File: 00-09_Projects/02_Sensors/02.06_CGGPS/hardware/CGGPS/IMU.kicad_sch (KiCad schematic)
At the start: 12 parts, among them U3 BNO086, Y1 Crystal_GND24

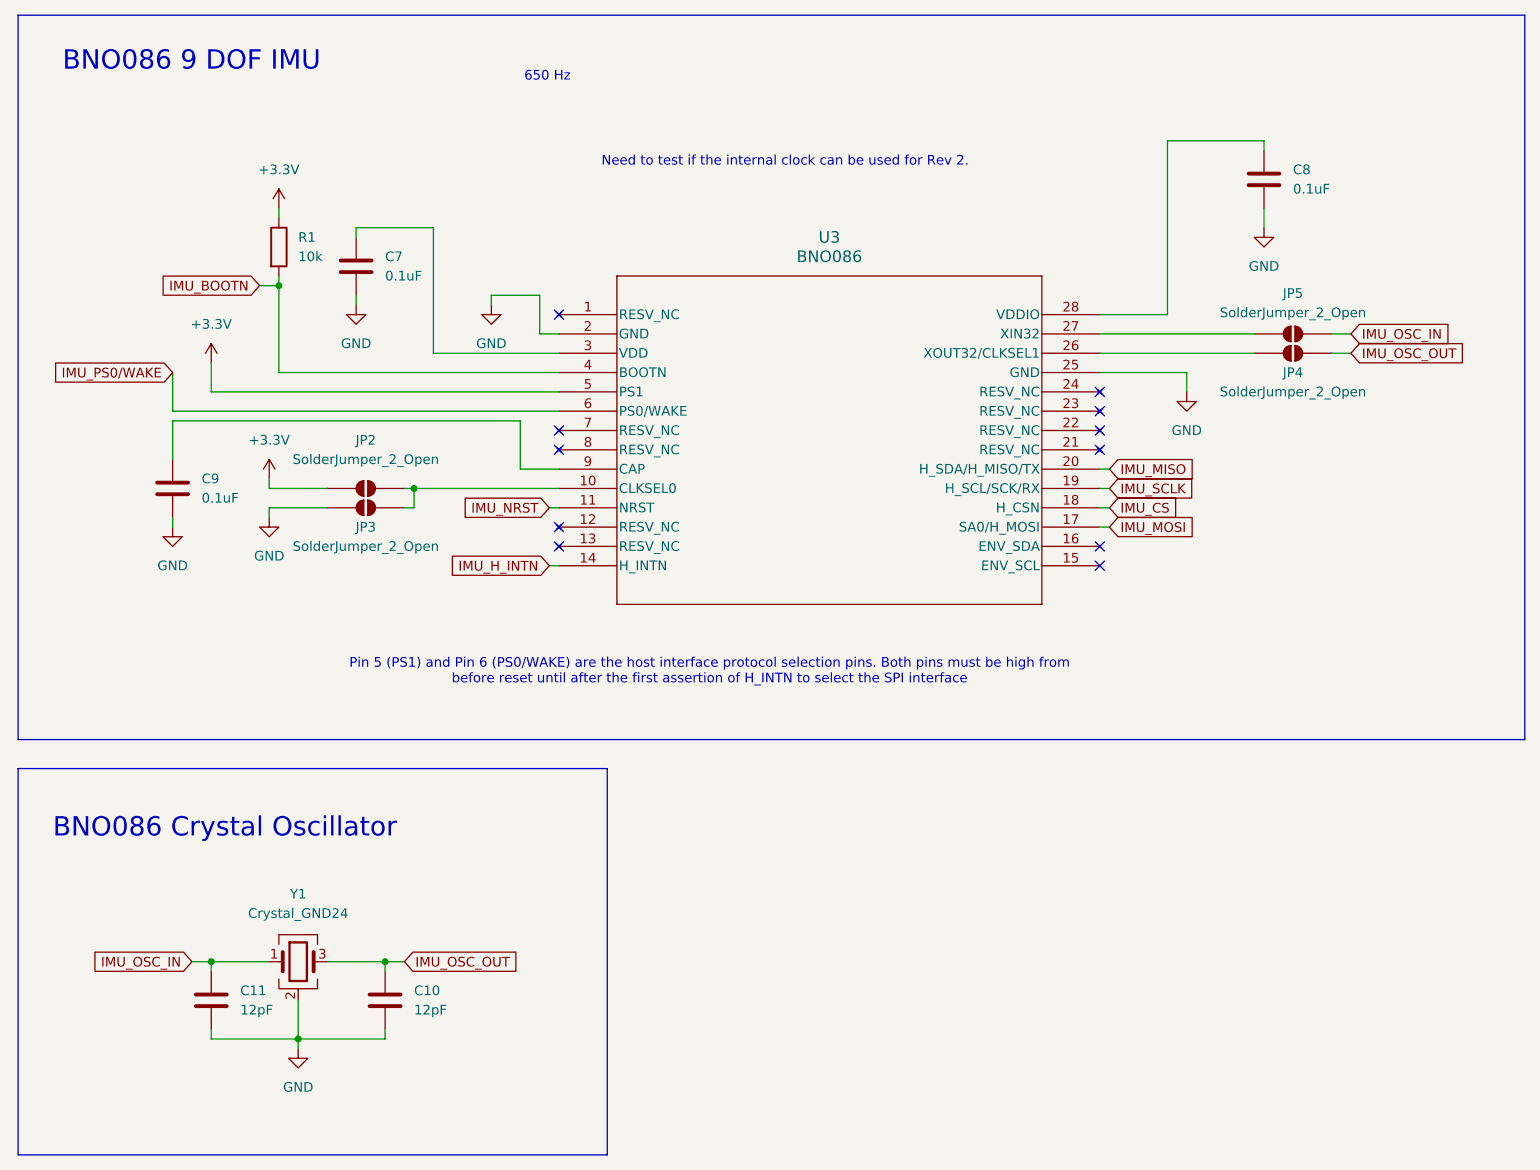
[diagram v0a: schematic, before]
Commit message: wip
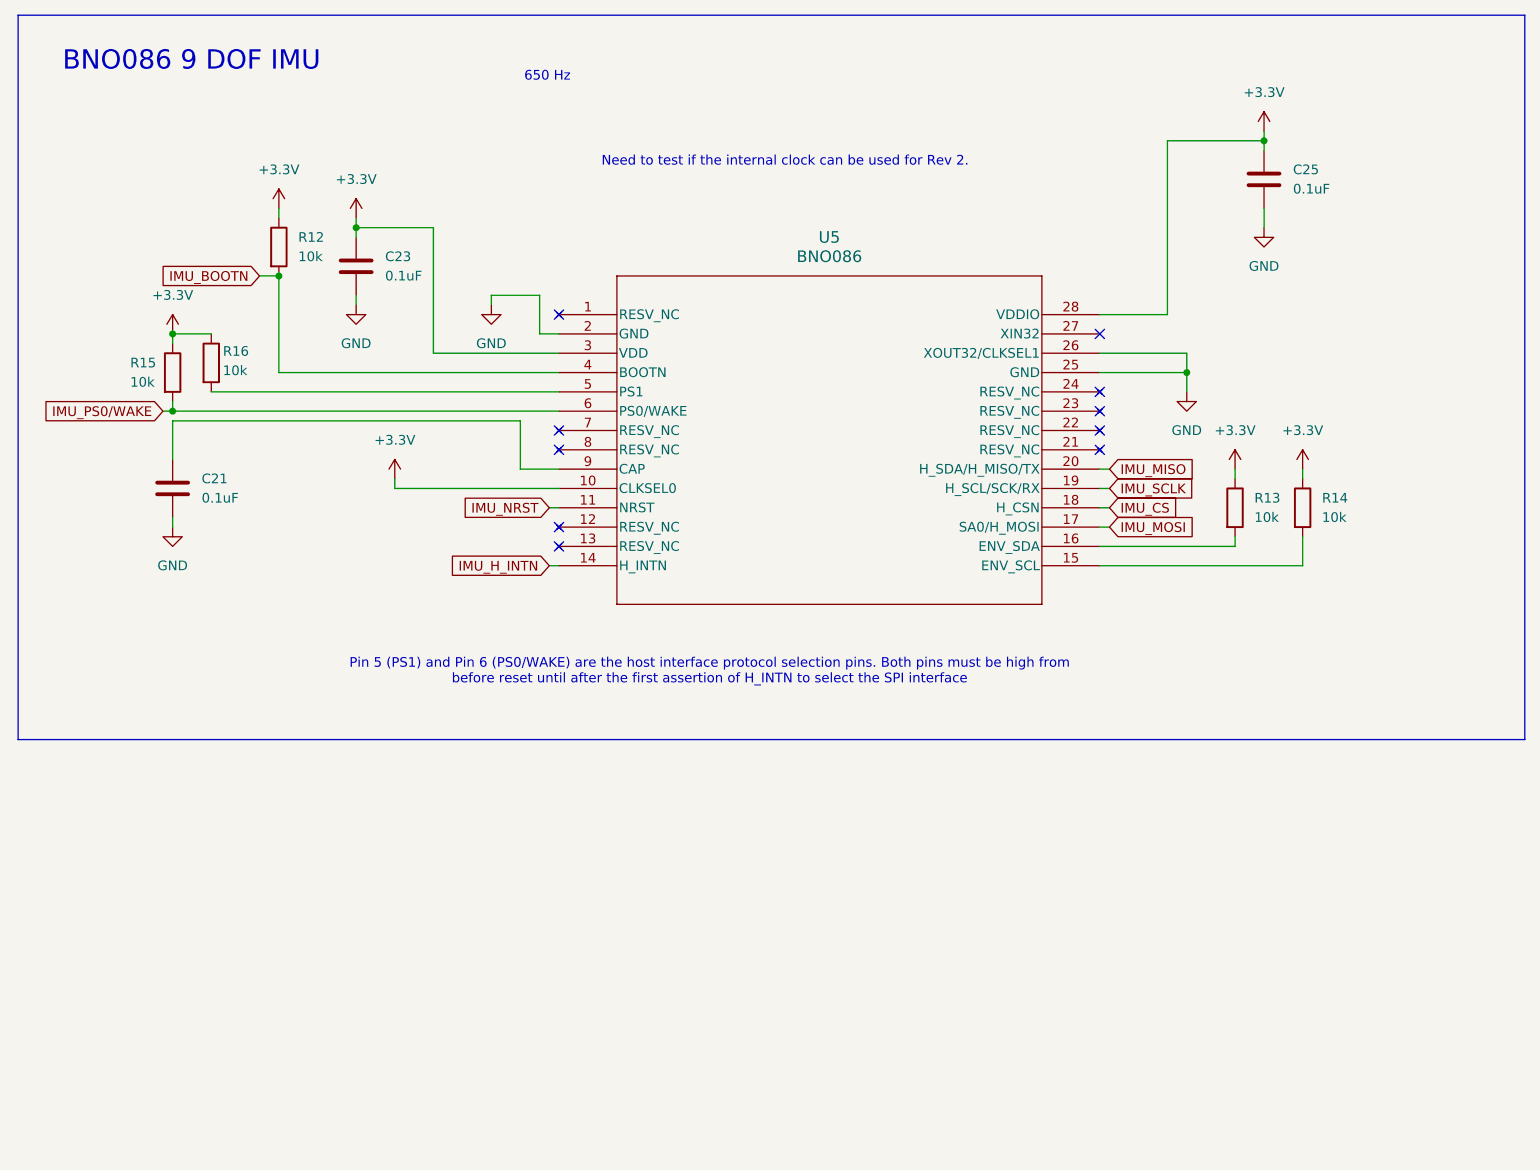
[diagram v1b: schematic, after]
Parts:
- removed C10, C11: 12pF, symbol Device:C
- removed JP2, JP3, JP4, JP5: SolderJumper_2_Open, symbol Jumper:SolderJumper_2_Open
- removed Y1: Crystal_GND24, symbol Device:Crystal_GND24
- added R13, R14, R15, R16: 10k, symbol Device:R
- renumbered C9 to C21, C7 to C23, C8 to C25, R1 to R12, U3 to U5
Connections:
- net +3.3V: now also C23.1, C25.1, U5.10 (CLKSEL0), U5.28 (VDDIO), U5.3 (VDD), R13.1, R14.1, R15.1, R16.1; no longer U5.5 (PS1)
- net GND: now also U5.26 (XOUT32/CLKSEL1)
- net IMU_PS0/WAKE: now also R15.2
- net at U5.15 (ENV_SCL): now also R14.2
- net at U5.16 (ENV_SDA): now also R13.2
- new net: R16.2, U5.5 (PS1)
- no-connect marks 11 -> 10
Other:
- note removed: "BNO086 Crystal Oscillator"
